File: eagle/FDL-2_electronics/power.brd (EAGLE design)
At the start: 37.8 x 25.4 mm, 6 parts, among them X1 JST-XH-02-PIN-ROUND-PAD, X2 JST-XH-02-PIN-ROUND-PAD

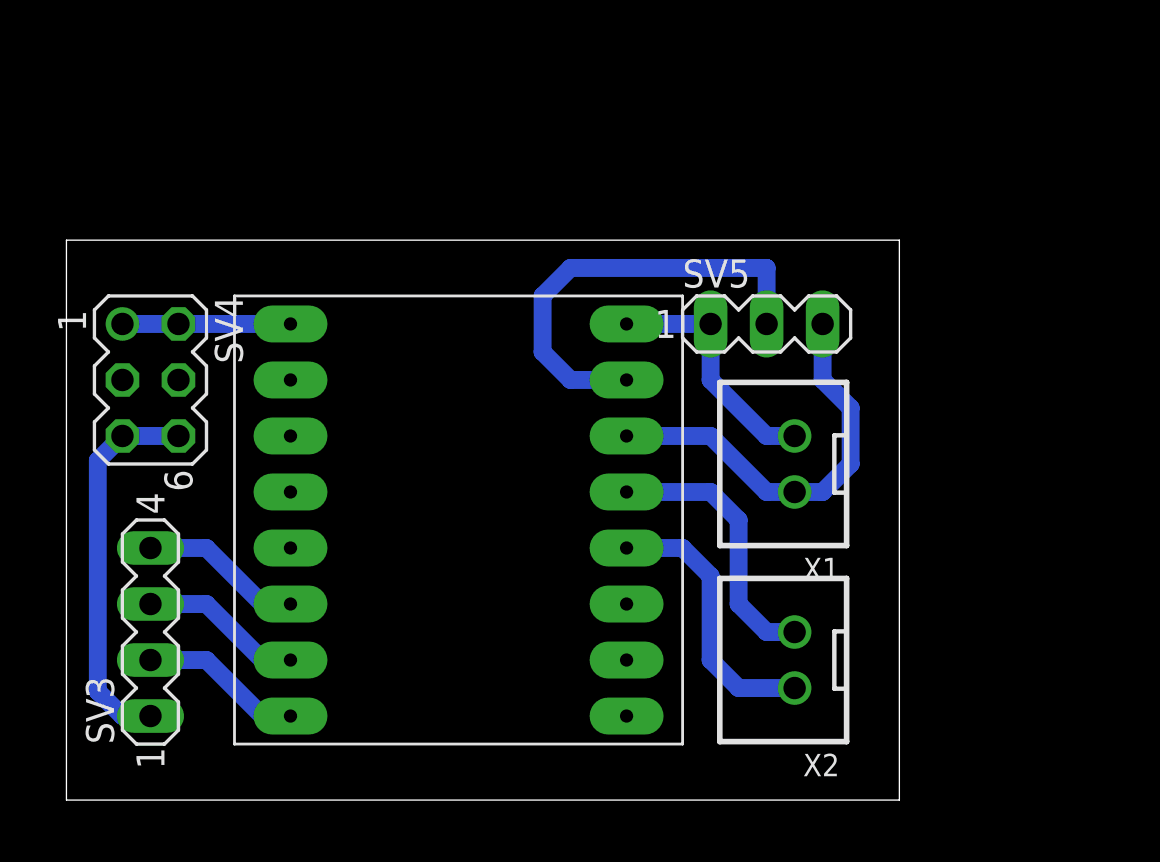
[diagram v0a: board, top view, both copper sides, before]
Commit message: some changes
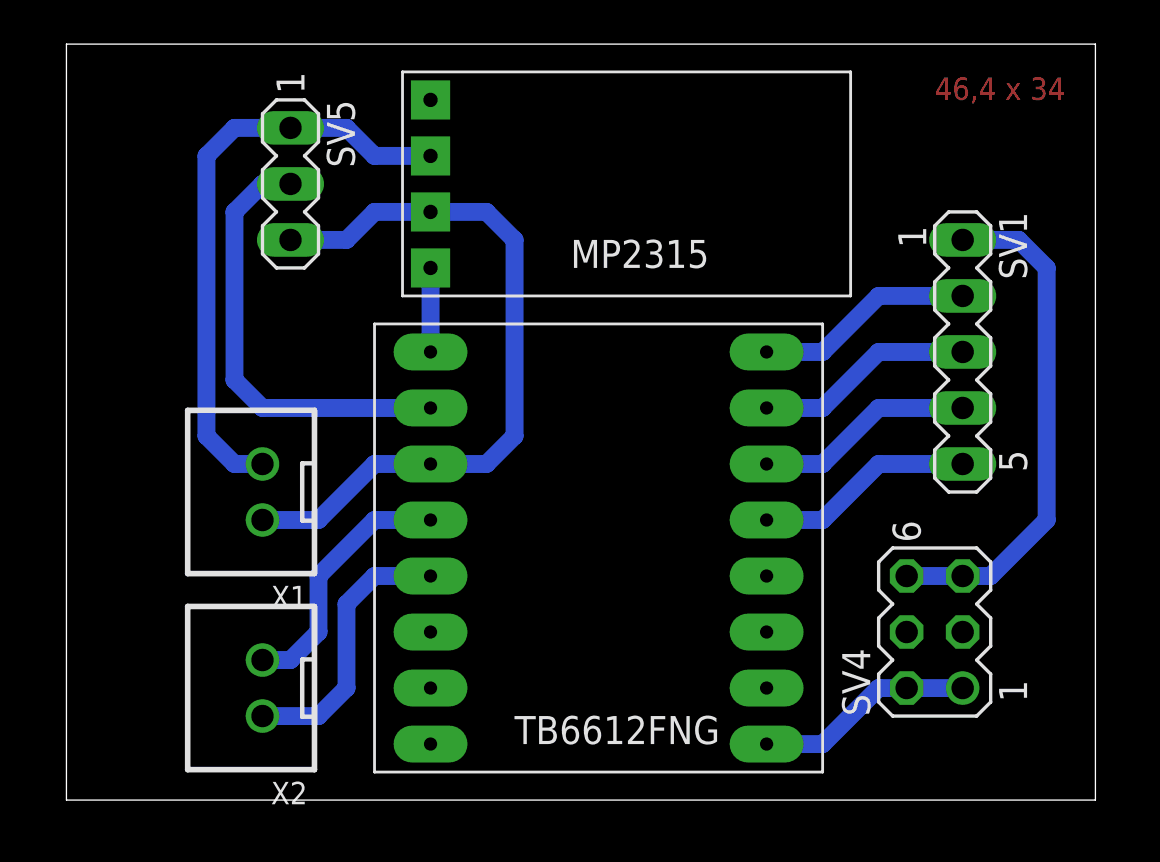
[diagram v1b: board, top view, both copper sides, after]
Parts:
- removed SV3: (no value), con-lstb:MA04-1
- added SV1: (no value), con-lstb:MA05-1
- added U$1: MP2315, mylib:MP2315
- moved SV4 37.4 mm to (39.4, 7.62), turned to 90 degrees
- moved X1 24.2 mm to (8.89, 14.0)
- moved X2 24.2 mm to (8.89, 5.08)
- moved SV5 22.5 mm to (10.2, 27.9), turned to 270 degrees
- moved U$2 7.41 mm to (24.1, 10.2), turned to 0 degrees
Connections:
- new net N$5: SV5.3, U$1.P$2, U$2.P$3, X1.1
- new net N$6: SV1.5, U$2.P$13
- net N$14: now also SV1.2, U$2.P$16; no longer SV3.2, U$2.P$9
- net N$21: now also SV1.3, U$2.P$15; no longer SV3.3, U$2.P$10
- net N$22: now also SV1.4, U$2.P$14; no longer SV3.4, U$2.P$11
- net N$24: now also U$2.P$9; no longer U$2.P$16
- net N$25: now also SV1.1; no longer SV3.1
- net N$3: now also U$1.P$1, U$2.P$1; no longer SV5.3, U$2.P$3, X1.1
- net N$4: now also U$1.P$3; no longer U$2.P$1
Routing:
- net N$5: track 0.00 -> 33.1 mm
- net N$4: track 11.2 -> 27.0 mm
- net N$3: track 18.6 -> 3.81 mm
- net N$6: track 0.00 -> 9.94 mm
- net N$25: track 17.4 -> 23.2 mm
- net N$22: track 7.40 -> 9.94 mm
- net N$14: track 7.40 -> 9.94 mm
- net N$21: track 7.40 -> 9.94 mm
- net N$24: track 7.62 -> 9.94 mm
- net N$1: track 12.5 -> 11.7 mm
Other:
- board size 37.8 x 25.4 mm -> 46.7 x 34.3 mm
- board text added: "46,4 x 34"
